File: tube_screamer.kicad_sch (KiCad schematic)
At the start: 53 parts, among them Q1 MMBT5551, Q2 MMBT5551, Q3 MMBT5551, U1 NE5532

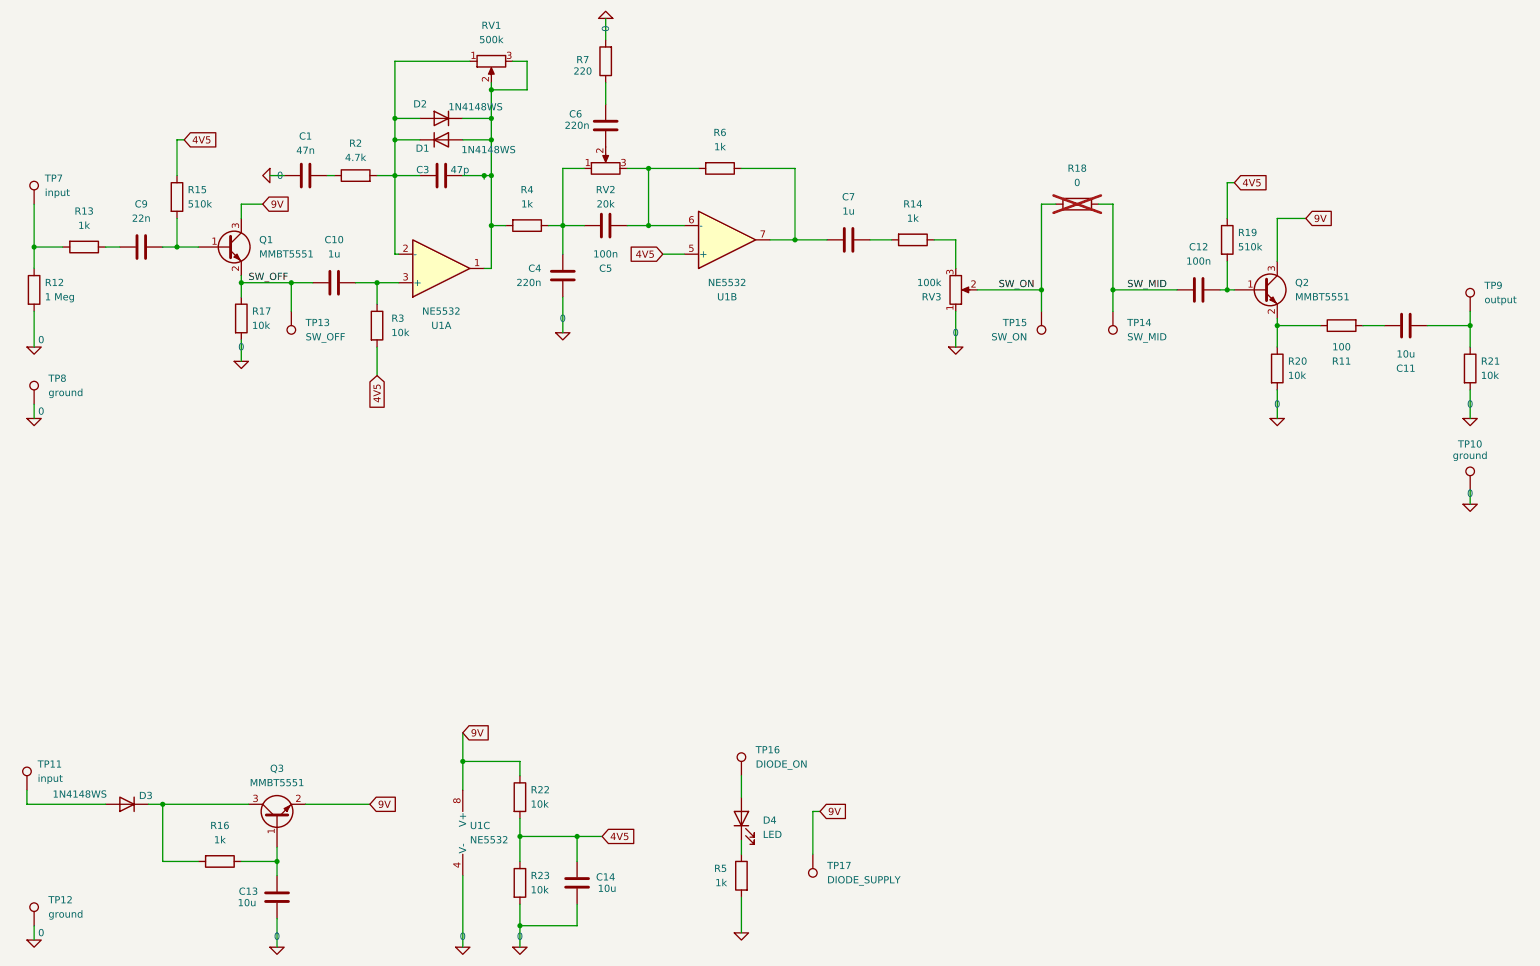
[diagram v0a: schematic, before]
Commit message: Idk
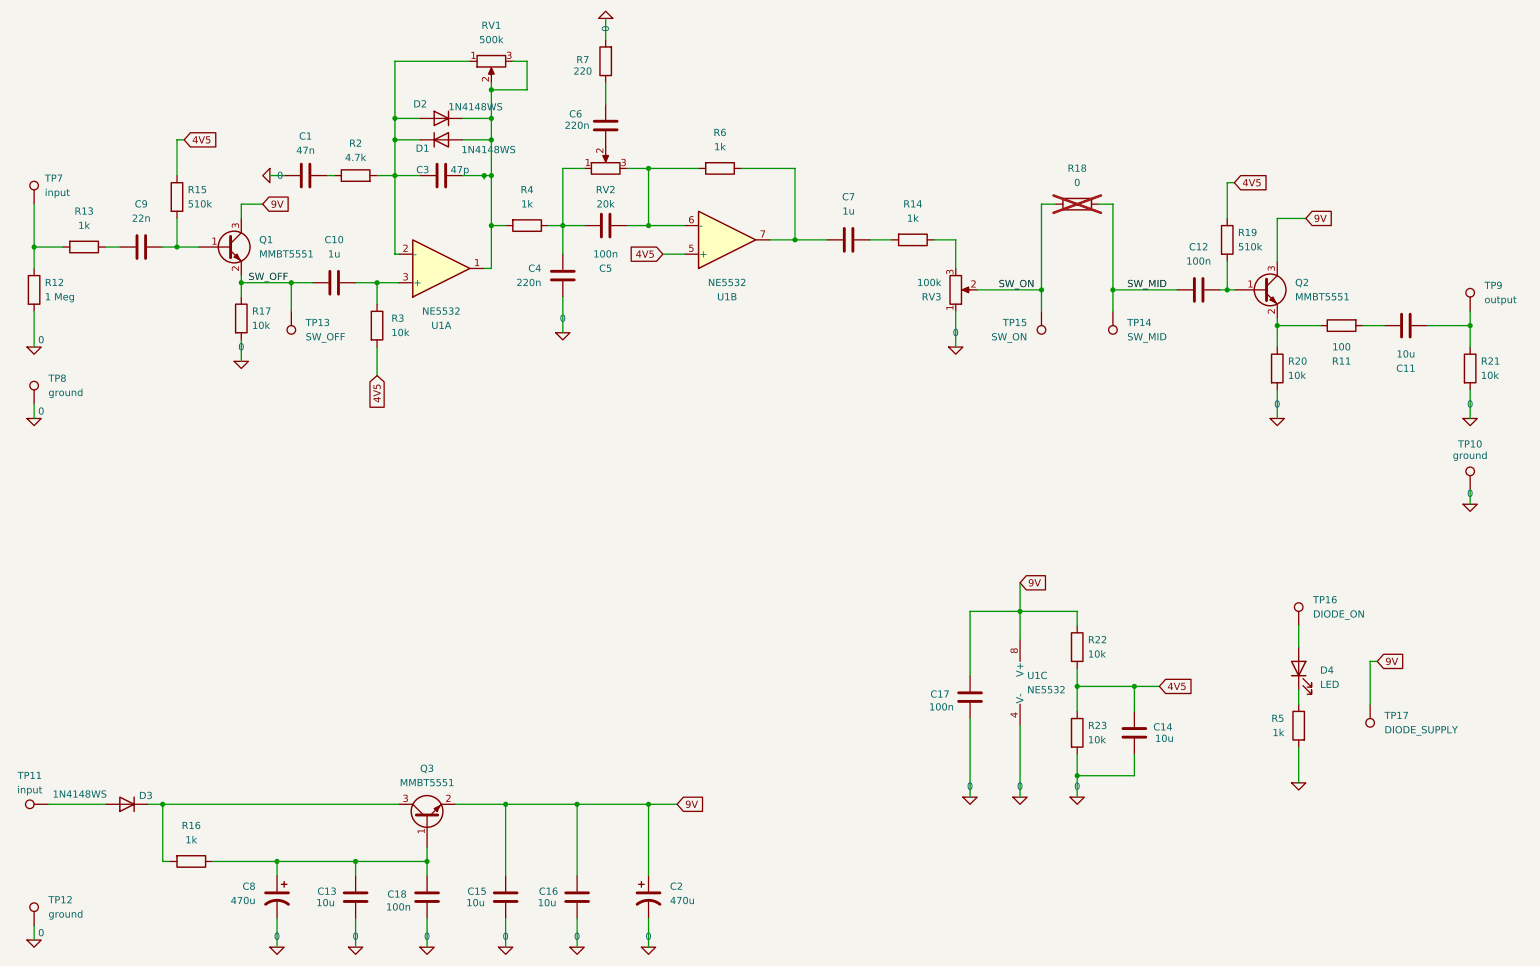
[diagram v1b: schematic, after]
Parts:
- added C15, C16: 10u, Capacitor_SMD:C_0603_1608Metric_Pad1.08x0.95mm_HandSolder, symbol Device:C
- added C17, C18: 100n, Capacitor_SMD:C_0603_1608Metric_Pad1.08x0.95mm_HandSolder, symbol Device:C
- added C2, C8: 470u, Capacitor_THT:CP_Radial_D8.0mm_P3.50mm, symbol Device:C_Polarized_US
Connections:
- net 0: now also C15.2, C16.2, C17.1, C18.1, C2.2, C8.2
- net 9V: now also C15.1, C16.1, C17.2, C2.1
- net at C13.1, Q3.1 (B), R16.1: now also C18.2, C8.1
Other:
- moved on the sheet: C13, C14, D4, Q3, R16, R22, R23, R5, TP11, TP16, TP17, U1C
